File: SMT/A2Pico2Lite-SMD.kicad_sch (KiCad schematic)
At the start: 56 parts, among them J1 SolderJumper_2_Bridged, SW1 SW_BOOTSEL, U1 RP2354A-QFN60, U2 ME6211, X1 ABM8-272-T3 12MHz

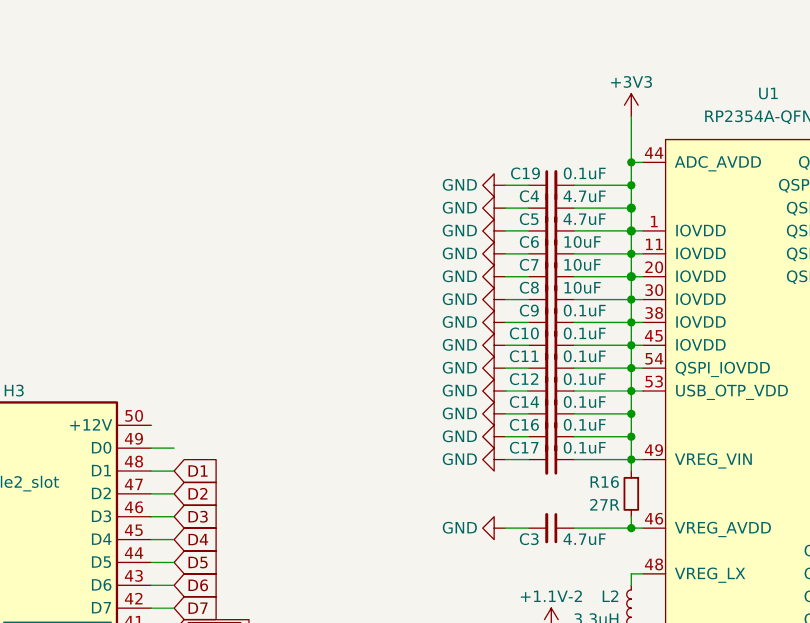
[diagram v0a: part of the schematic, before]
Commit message: Add files via upload
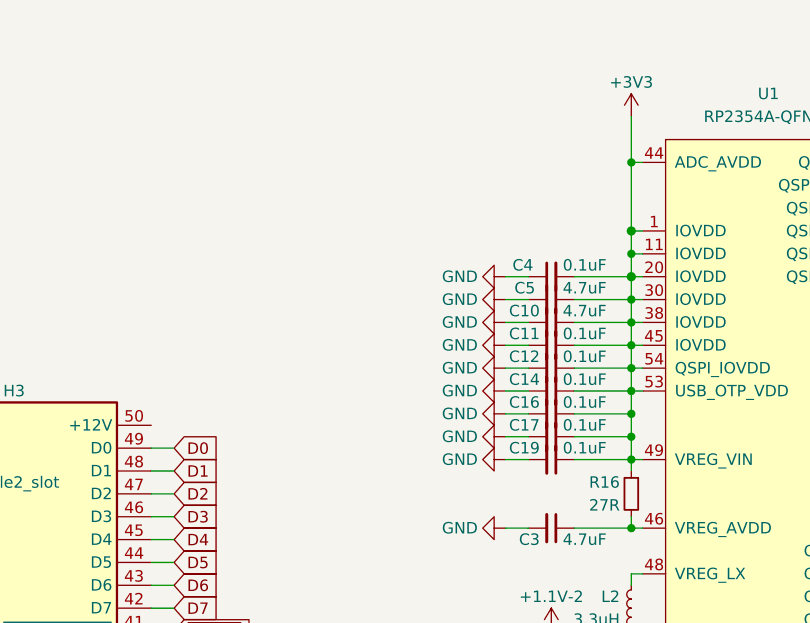
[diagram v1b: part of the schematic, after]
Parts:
- removed C6, C7, C8: 10uF, Capacitor_SMD:C_0603_1608Metric, symbol Device:C_Small
- removed C9: 0.1uF, Capacitor_SMD:C_0603_1608Metric, symbol Device:C_Small
- renumbered C5 to C10, C10 to C11, C11 to C12, C12 to C14, C14 to C16, C16 to C17, C17 to C19, C19 to C4, C4 to C5
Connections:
- net D0: now also H3.49 (D0)
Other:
- moved on the sheet: C10, C4, C5

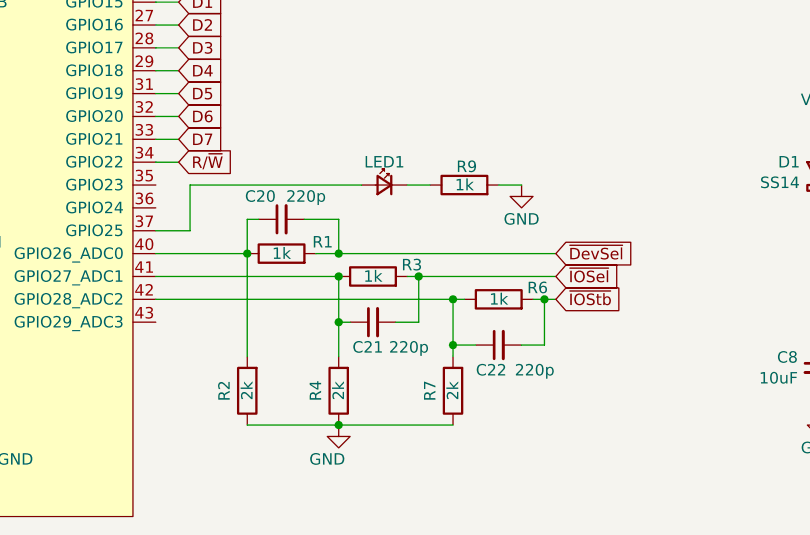
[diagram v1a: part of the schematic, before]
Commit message: Add files via upload
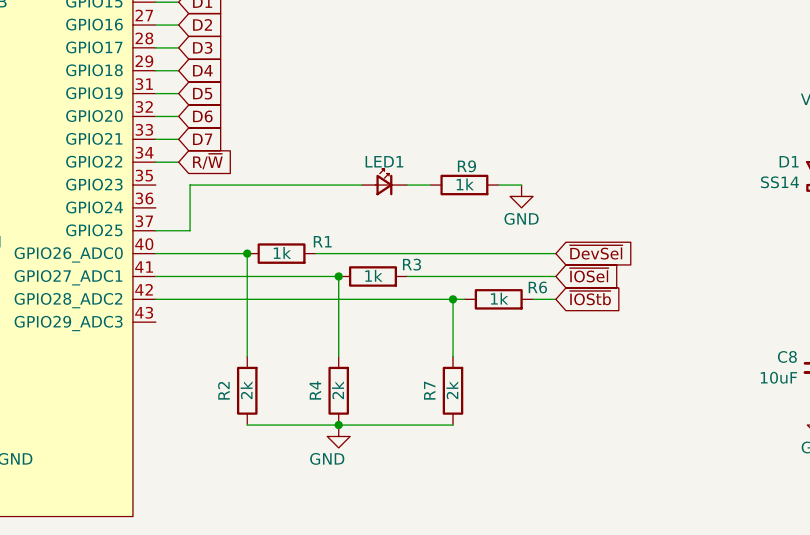
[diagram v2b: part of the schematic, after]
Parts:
- removed C20, C21, C22: 220p, Capacitor_SMD:C_0603_1608Metric, symbol Device:C_Small
